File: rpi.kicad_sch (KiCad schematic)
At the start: 10 parts, among them J10 RPI, J11 SERIAL, J12 I2C, J13 LCD, Q23 2N7002K, Q24 2N7002K

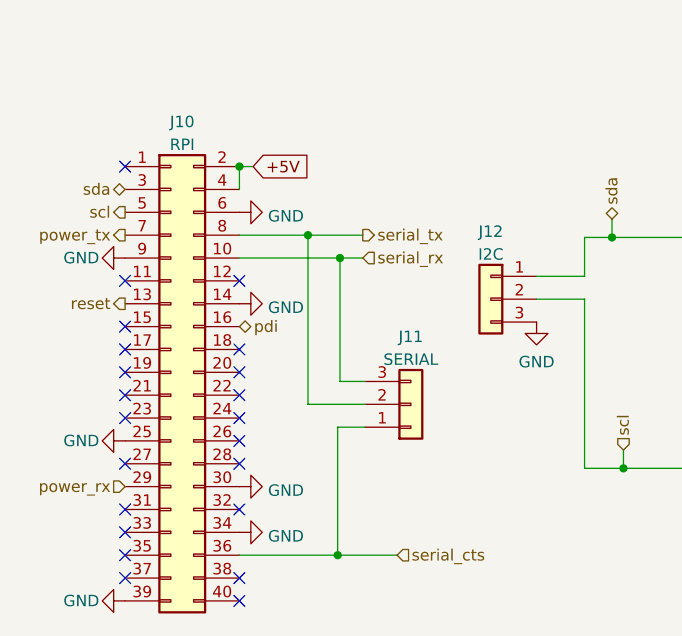
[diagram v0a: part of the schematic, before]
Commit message: put all schematics on 50 mil grid
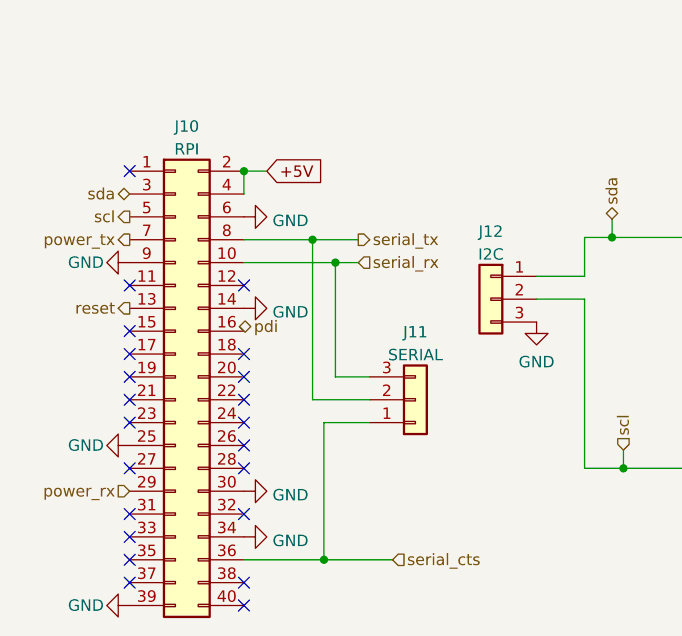
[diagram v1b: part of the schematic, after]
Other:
- moved on the sheet: J10, J11

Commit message: minor corrections in prep for new build
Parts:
- J11, J12: Model Do Not Populate -> 68001-403HLF
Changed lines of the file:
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@@
       (effects (font (size 1.27 1.27)) hide)
     )
-    (property "Model" "Do Not Populate" (id 4) (at 96.52 116.84 0)
+    (property "Model" "68001-403HLF" (id 4) (at 96.52 116.84 0)
       (effects (font (size 1.27 1.27)) hide)
     )
@@
       (effects (font (size 1.27 1.27)) hide)
     )
-    (property "Model" "Do Not Populate" (id 4) (at 104.902 105.664 0)
+    (property "Model" "68001-403HLF" (id 4) (at 104.902 105.664 0)
       (effects (font (size 1.27 1.27)) hide)
     )
